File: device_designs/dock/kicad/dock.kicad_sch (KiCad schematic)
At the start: 21 parts, among them J1 USB4085, J2A USB4085, J2B USB4085, J3A USB3_A, J3B USB3_A, J4 HDMI_TypeA, J5 JK0-0136NL, J6 Mill-Max_pogo, U1 JHL8440, U1A VL108, U1R JHL9040R, U2 TPS65994ADFBRQ1, U3 RTL8156, U4 VL817, U5 TPS55288RPMR, U6 TPS62864, U7 TLV75533PDRVR, U8 DWM3001C, U9 ALC4050

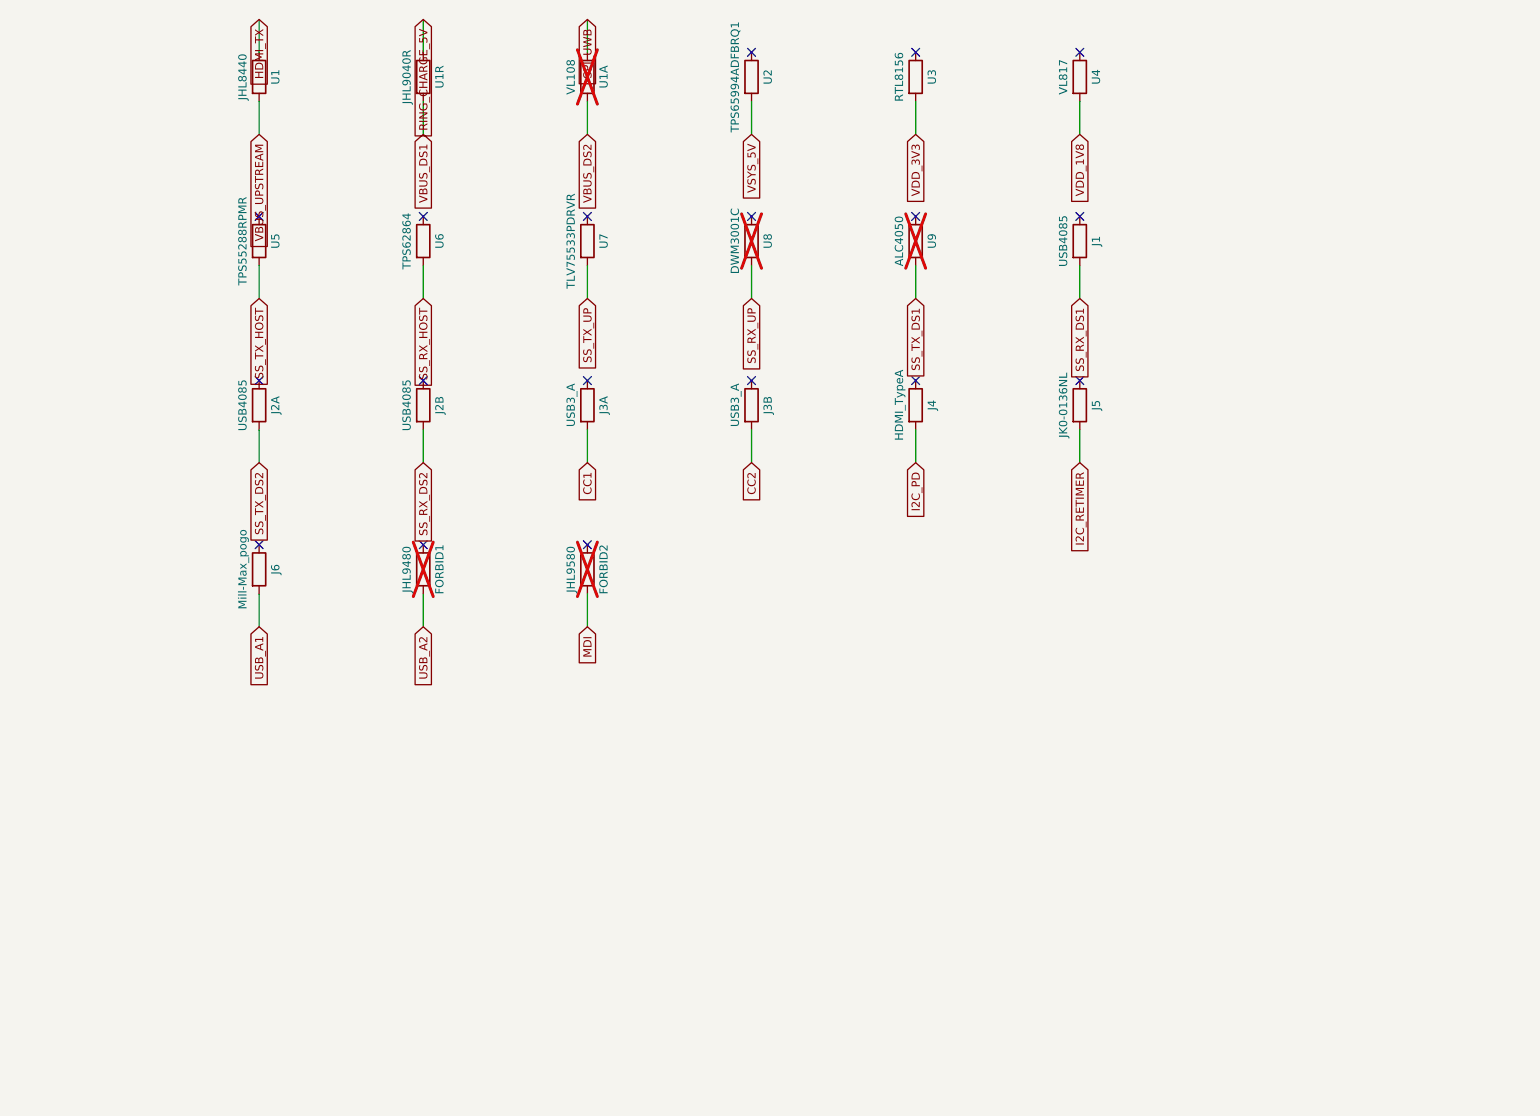
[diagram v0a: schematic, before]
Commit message: feat(eda): Continuation VIII manufacturer release packages for five-product family
Expand beyond Cont VII FuncBlock placeholders to multi-pin functional circuits with exact MPNs, power trees, routed PCBs, and digital manufacturing packages. Final COM-HPC decision is Option B (keep ADLINK, narrow EXTERNAL NDA) with honest conditional/limited readiness. ERC/DRC errors are zero on all five boards under KiCad 10.0.5; PHYSICAL_EXECUTION_FREEZE remains active.

Co-authored-by: Cursor <cursoragent@cursor.com>
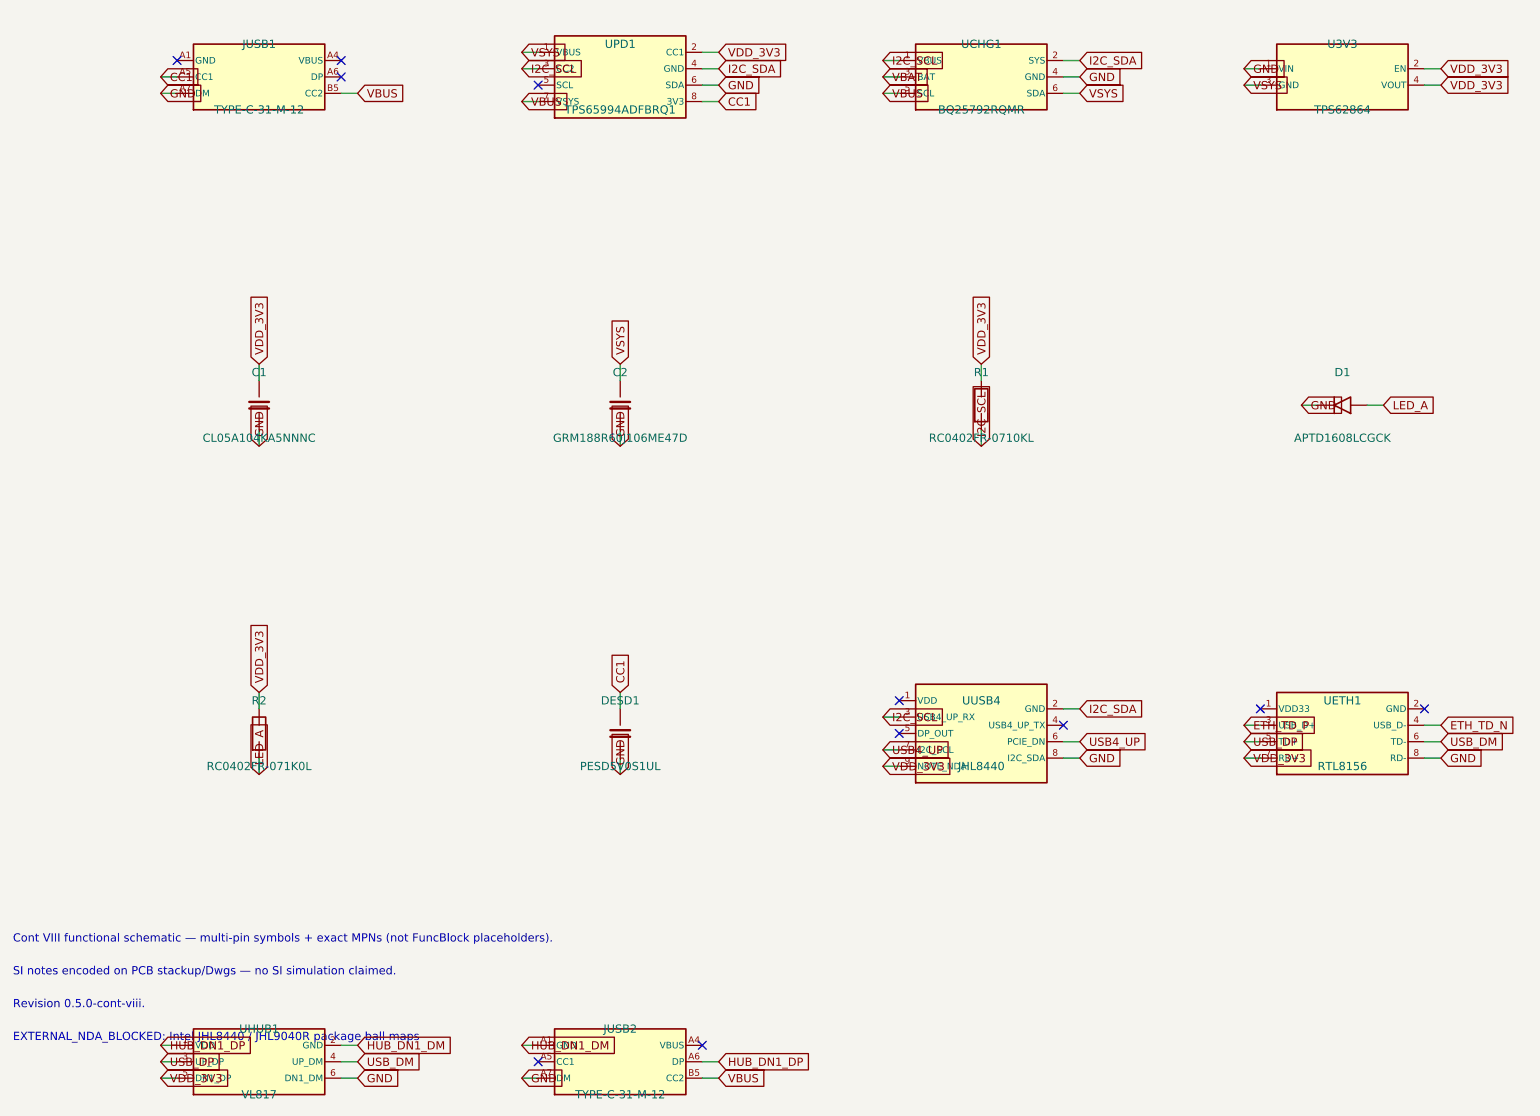
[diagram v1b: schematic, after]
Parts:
- removed FORBID1: JHL9480, gunnchos_structural:Block_SMD_10x10, symbol FuncBlock
- removed FORBID2: JHL9580, gunnchos_structural:Block_SMD_10x10, symbol FuncBlock
- removed J1, J2A, J2B: USB4085, gunnchos_structural:Block_SMD_10x10, symbol FuncBlock
- removed J3A, J3B: USB3_A, gunnchos_structural:Block_SMD_10x10, symbol FuncBlock
- removed J4: HDMI_TypeA, gunnchos_structural:Block_SMD_10x10, symbol FuncBlock
- removed J5: JK0-0136NL, gunnchos_structural:Block_SMD_10x10, symbol FuncBlock
- removed J6: Mill-Max_pogo, gunnchos_structural:Block_SMD_10x10, symbol FuncBlock
- removed U1: JHL8440, gunnchos_structural:Block_SMD_10x10, symbol FuncBlock
- removed U1A: VL108, gunnchos_structural:Block_SMD_10x10, symbol FuncBlock
- removed U1R: JHL9040R, gunnchos_structural:Block_SMD_10x10, symbol FuncBlock
- removed U2: TPS65994ADFBRQ1, gunnchos_structural:Block_SMD_10x10, symbol FuncBlock
- removed U3: RTL8156, gunnchos_structural:Block_SMD_10x10, symbol FuncBlock
- removed U4: VL817, gunnchos_structural:Block_SMD_10x10, symbol FuncBlock
- removed U5: TPS55288RPMR, gunnchos_structural:Block_SMD_10x10, symbol FuncBlock
- removed U6: TPS62864, gunnchos_structural:Block_SMD_10x10, symbol FuncBlock
- removed U7: TLV75533PDRVR, gunnchos_structural:Block_SMD_10x10, symbol FuncBlock
- removed U8: DWM3001C, gunnchos_structural:Block_SMD_10x10, symbol FuncBlock
- removed U9: ALC4050, gunnchos_structural:Block_SMD_10x10, symbol FuncBlock
- added C1: CL05A104KA5NNNC, gunnchos_functional:C_0402, symbol C
- added C2: GRM188R60J106ME47D, gunnchos_functional:C_0402, symbol C
- added D1: APTD1608LCGCK, gunnchos_functional:LED_0603, symbol LED
- added DESD1: PESD5V0S1UL, gunnchos_functional:R_0402, symbol C
- added JUSB1, JUSB2: TYPE-C-31-M-12, gunnchos_functional:Block_SMD_safe, symbol USB_C
- added R1: RC0402FR-0710KL, gunnchos_functional:R_0402, symbol R
- added R2: RC0402FR-071K0L, gunnchos_functional:R_0402, symbol R
- added U3V3: TPS62864, gunnchos_functional:Block_SMD_safe, symbol BUCK
- added UCHG1: BQ25792RQMR, gunnchos_functional:Block_SMD_safe, symbol CHARGER
- added UETH1: RTL8156, gunnchos_functional:Block_SMD_safe, symbol RTL8156
- added UHUB1: VL817, gunnchos_functional:Block_SMD_safe, symbol VL817
- added UPD1: TPS65994ADFBRQ1, gunnchos_functional:Block_SMD_safe, symbol PD_CTRL
- added UUSB4: JHL8440, gunnchos_functional:Block_SMD_safe, symbol JHL8440_ROLE
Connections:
- net CC1: now also DESD1.1, JUSB1.A5 (CC1), UPD1.8 (3V3)
- net VDD_3V3: now also C1.1, R1.1, R2.1, U3V3.2 (EN), U3V3.4 (VOUT), UETH1.7 (RD+), UHUB1.5 (DN1_DP), UPD1.2 (CC1), UUSB4.9 (NOTE_NDA)
- new net ETH_TD_N: UETH1.4 (USB_D-)
- new net ETH_TD_P: UETH1.3 (USB_D+)
- new net GND: C1.2, C2.2, D1.1 (K), DESD1.2, JUSB1.A7 (DM), JUSB2.A7 (DM), U3V3.1 (VIN), UCHG1.4 (GND), UETH1.8 (RD-), UHUB1.6 (DN1_DM), UPD1.6 (SDA), UUSB4.8 (I2C_SDA)
- new net HUB_DN1_DM: JUSB2.A1 (GND), UHUB1.2 (GND)
- new net HUB_DN1_DP: JUSB2.A6 (DP), UHUB1.1 (VDD)
- new net I2C_SCL: R1.2, UCHG1.1 (VBUS), UPD1.3 (CC2), UUSB4.3 (USB4_UP_RX)
- new net I2C_SDA: UCHG1.2 (SYS), UPD1.4 (GND), UUSB4.2 (GND)
- new net LED_A: D1.2 (A), R2.2
- new net USB4_UP: UUSB4.6 (PCIE_DN), UUSB4.7 (I2C_SCL)
- new net USB_DM: UETH1.6 (TD-), UHUB1.4 (UP_DM)
- new net USB_DP: UETH1.5 (TD+), UHUB1.3 (UP_DP)
- new net VBAT: UCHG1.3 (BAT)
- new net VBUS: JUSB1.B5 (CC2), JUSB2.B5 (CC2), UCHG1.5 (SCL), UPD1.7 (VSYS)
- new net VSYS: C2.1, U3V3.3 (GND), UCHG1.6 (SDA), UPD1.1 (VBUS)
- no-connect marks 18 -> 11
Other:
- note added: "Cont VIII functional schematic — multi-pin symbols + exact MPNs (not FuncBlock placeholders)."
- note added: "EXTERNAL_NDA_BLOCKED: Intel JHL8440 / JHL9040R package ball maps"
- note added: "Revision 0.5.0-cont-viii."
- note added: "SI notes encoded on PCB stackup/Dwgs — no SI simulation claimed."
- company: gunnchOS3k / CONTINUATION VII -> gunnchOS3k / CONTINUATION VIII
- title: Dock Main PCB — USB4/TB4 Cont VII -> Dock Main PCB — USB4/TB4 Cont VIII
